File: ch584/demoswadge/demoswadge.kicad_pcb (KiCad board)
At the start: 2 copper layers, 10.7 x 10.7 mm, 86 parts, among them J1 SAO, J2 PJ-307C, P1 USB_C_Plug_USB2.0, Q1 PMOS, Q2 PMOS, SW1 TS-1187A-B-A-B, SW2 TS-1187A-B-A-B, SW3 TS-1187A-B-A-B, SW4 TS-1187A-B-A-B, SW5 TS-1187A-B-A-B, SW6 TS-1187A-B-A-B, SW7 TS-1187A-B-A-B, U2 SM5701_2.2V, U3 XC6206PxxxMR, U4 XT1861B332MR-G, U6 LSM6DSL, Y1 32MHz, Y2 32.768kHz

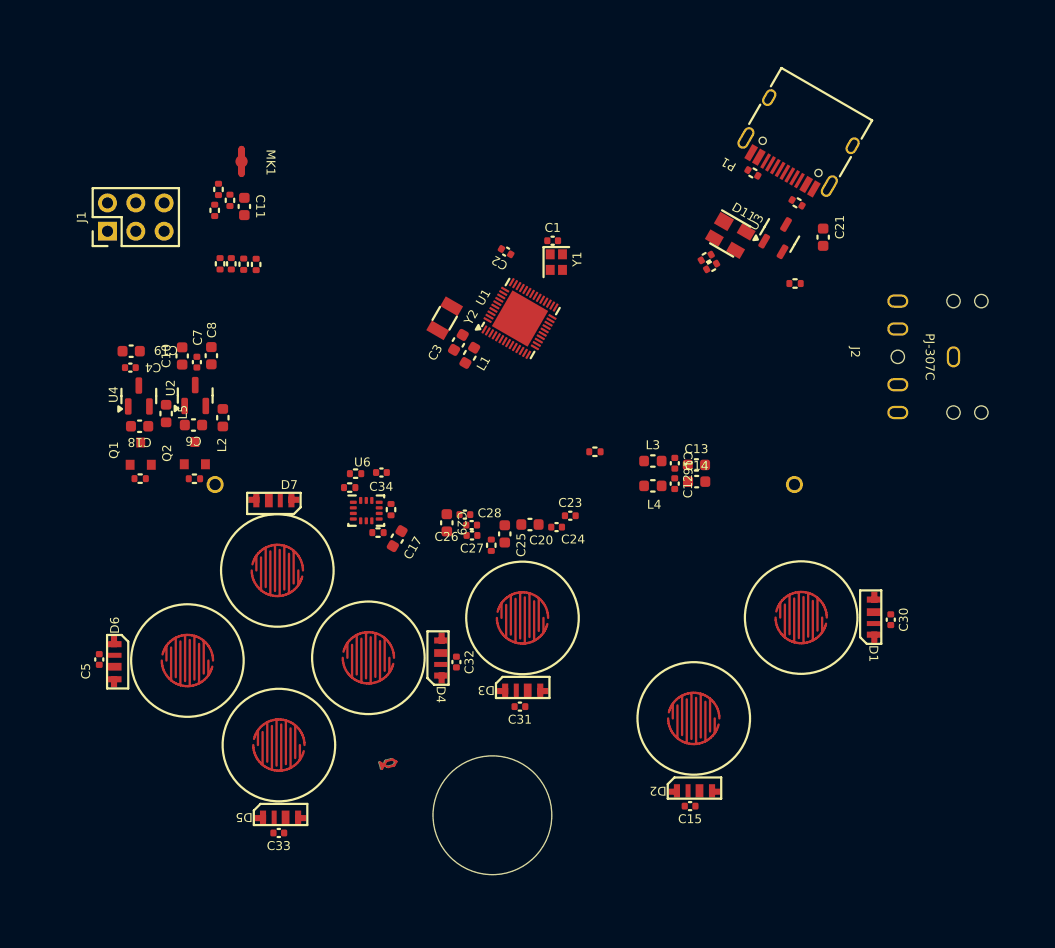
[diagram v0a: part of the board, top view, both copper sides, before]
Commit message: Bump demoswadge
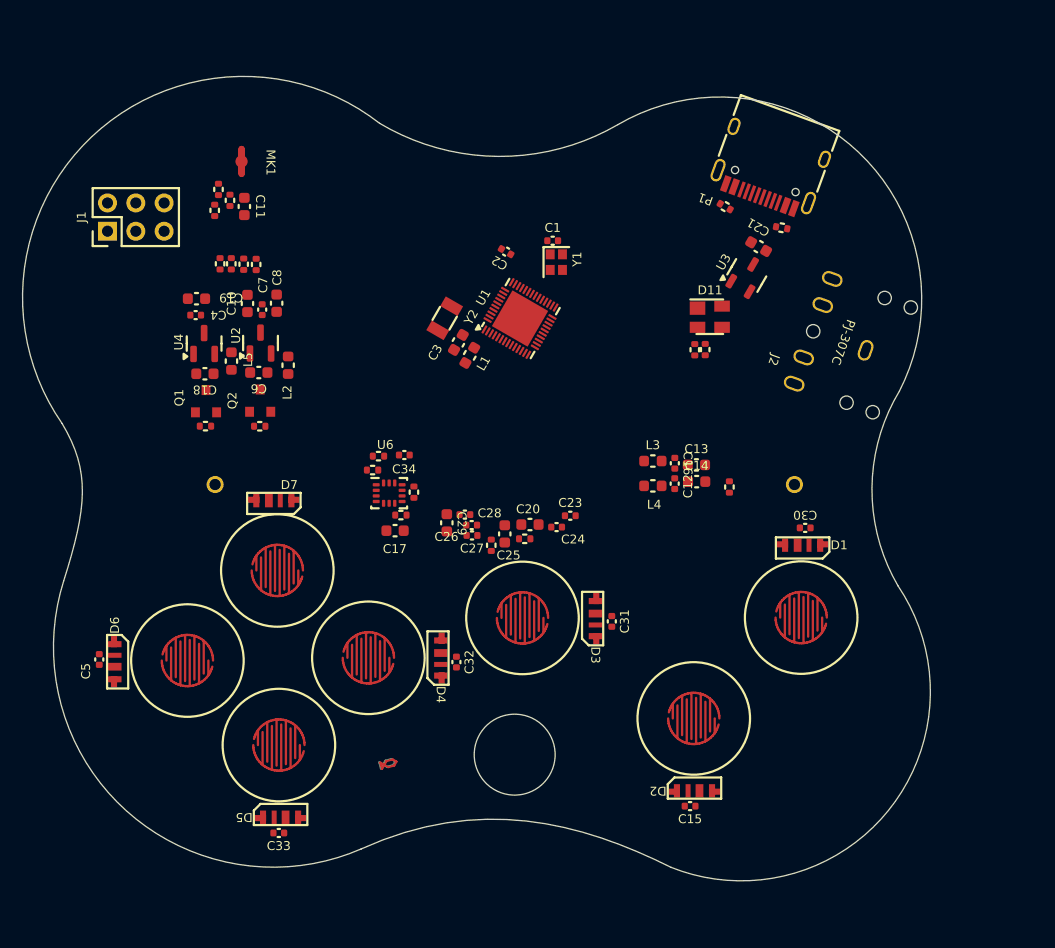
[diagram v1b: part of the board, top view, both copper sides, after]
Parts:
- moved R3 19.2 mm to (122.0, 108.5), turned to -90 degrees
- moved C30 11.3 mm to (128.8, 112.2), turned to 0 degrees
- moved C31 11.2 mm to (111.4, 120.6), turned to -90 degrees
- moved R15 10.0 mm to (103.6, 113.2)
- moved D3 9.16 mm to (110.0, 120.4), turned to -90 degrees
- moved D1 9.07 mm to (128.6, 113.8), turned to 0 degrees
- moved R14 8.34 mm to (118.9, 96.2), turned to 90 degrees
- moved J2 7.91 mm to (134.2, 96.3), turned to -110 degrees
- moved D11 7.56 mm to (120.2, 93.3), turned to 0 degrees
- moved C18 7.52 mm to (74.9, 98.4)
- moved C10 7.52 mm to (78.7, 92.1)
- moved C8 7.52 mm to (81.4, 92.1)
- moved L2 7.52 mm to (82.4, 97.6)
- moved Q1 7.52 mm to (75.0, 100.8)
- moved Q2 7.52 mm to (79.9, 100.8)
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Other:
- board size 10.7 x 10.7 mm -> 81.5 x 72.2 mm
